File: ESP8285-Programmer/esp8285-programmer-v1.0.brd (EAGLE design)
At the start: 38.2 x 15.2 mm, 30 parts, among them J1 6p-2.54, J2 2p-2.54, J3 2p-2.54, K1 B3U-1000P, Q1 S9013, Q2 S9013, U1 CH340T-SSOP20, U2 CJA1117B-3.3-SOT89, Y1 12MHZ

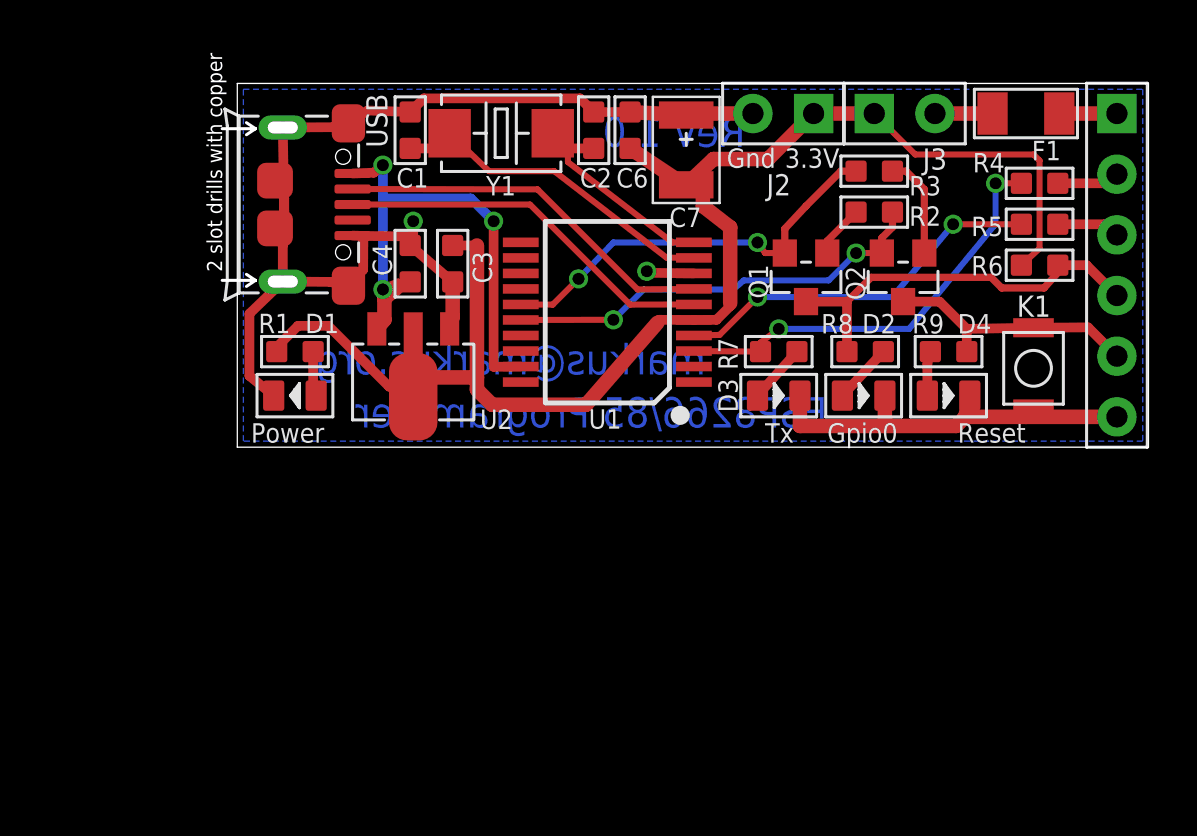
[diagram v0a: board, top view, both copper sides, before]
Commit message: Another Rev 1.0
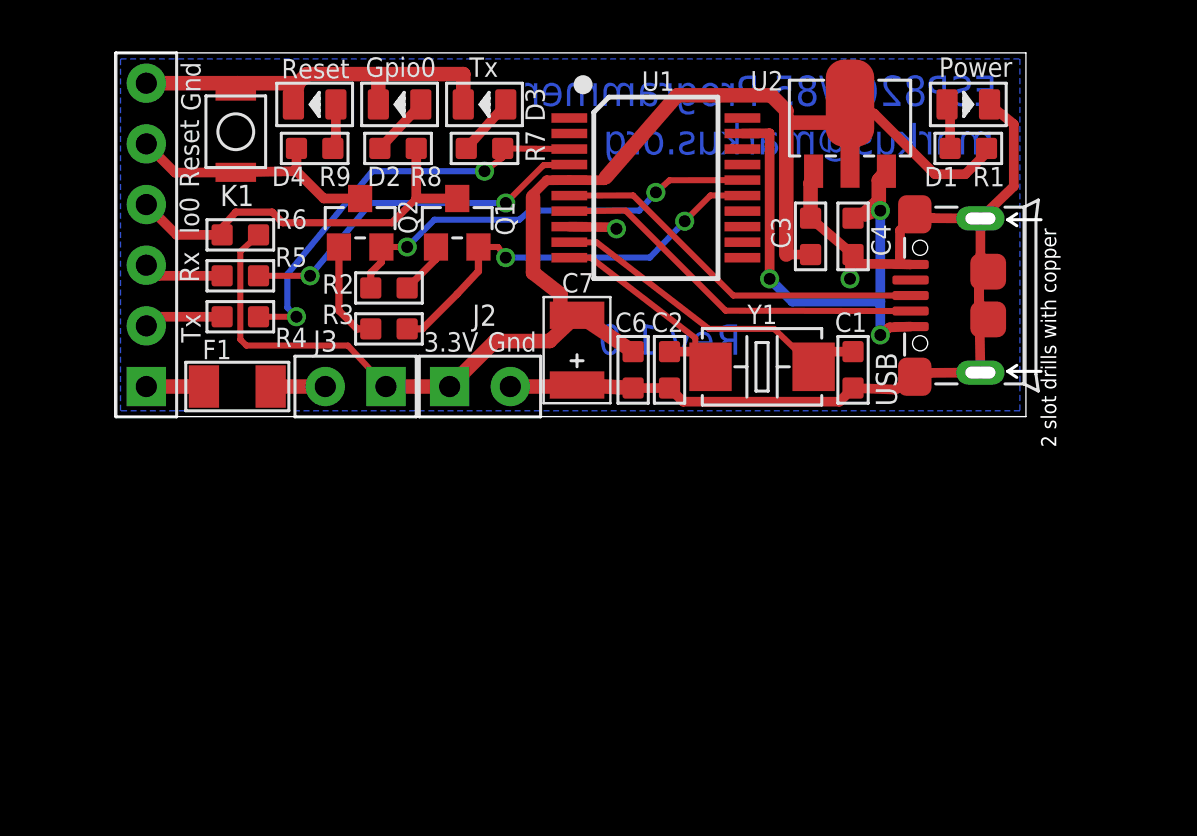
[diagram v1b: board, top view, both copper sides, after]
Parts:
- moved J1 40.7 mm to (2.54, 22.9), turned to 180 degrees
- moved F1 34.9 mm to (6.35, 16.5), turned to 0 degrees
- moved K1 34.8 mm to (6.29, 27.2), turned to 270 degrees
- moved R4 33.9 mm to (6.48, 19.4), turned to 270 degrees
- moved R5 33.5 mm to (6.48, 21.1), turned to 270 degrees
- moved R6 33.5 mm to (6.48, 22.9), turned to 270 degrees
- moved D1 30.7 mm to (37.0, 28.3), turned to 0 degrees
- moved R1 29.5 mm to (37.0, 26.5), turned to 90 degrees
- moved D4 29.2 mm to (9.59, 28.3), turned to 180 degrees
- moved R9 27.9 mm to (9.59, 26.5), turned to 270 degrees
- moved J3 25.7 mm to (11.3, 16.5), turned to 270 degrees
- moved USB 23.2 mm to (34.3, 20.3), turned to 90 degrees
- moved D2 22.9 mm to (13.1, 28.3), turned to 180 degrees
- moved Q2 22.8 mm to (11.5, 23.4), turned to 0 degrees
- moved R3 21.4 mm to (12.7, 18.9), turned to 90 degrees
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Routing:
- net N$15: track 2.64 -> 3.34 mm
- net N$14: track 2.59 -> 3.29 mm
- net N$RX: track 15.8 -> 15.1 mm
- net +3V3: track 63.0 -> 62.3 mm
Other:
- board text added: "Io0"
- board text added: "Rx"

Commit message: Hopefully final V1.0
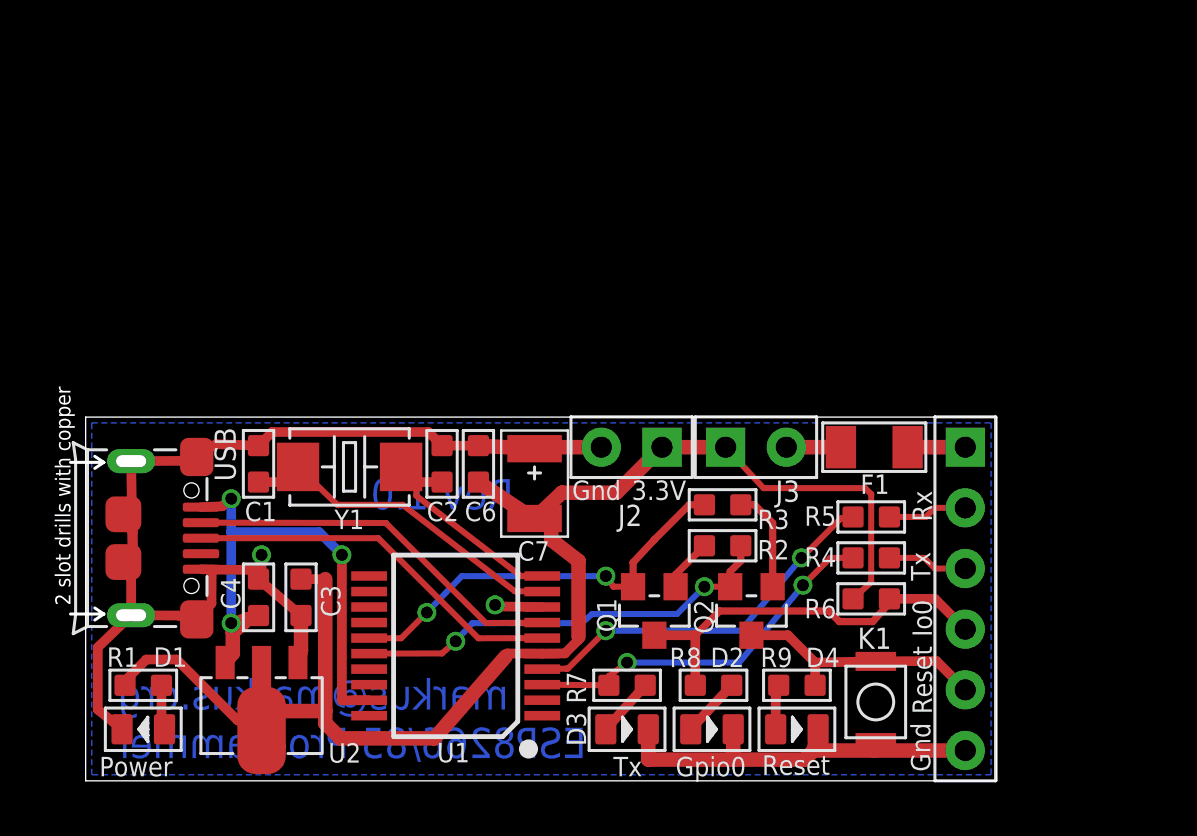
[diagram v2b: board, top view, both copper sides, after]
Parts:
- moved D1 43.3 mm to (2.41, 2.16), turned to 180 degrees
- moved R1 41.2 mm to (2.41, 4.00), turned to 270 degrees
- moved J1 37.5 mm to (36.8, 7.62), turned to 0 degrees
- moved K1 35.9 mm to (33.1, 3.30), turned to 90 degrees
- moved U2 34.7 mm to (7.37, 3.05), turned to 180 degrees
- moved D4 33.0 mm to (29.8, 2.16), turned to 0 degrees
- moved USB 30.9 mm to (5.08, 10.2), turned to 270 degrees
- moved R6 30.5 mm to (32.9, 7.62), turned to 90 degrees
- moved R9 30.2 mm to (29.8, 4.00), turned to 90 degrees
- moved D2 29.3 mm to (26.2, 2.16), turned to 0 degrees
- moved C4 29.1 mm to (7.24, 7.68), turned to 0 degrees
- moved R4 28.3 mm to (32.9, 9.33), turned to 90 degrees
- moved R5 28.3 mm to (32.9, 11.0), turned to 90 degrees
- moved D3 26.8 mm to (22.7, 2.16), turned to 0 degrees
- moved F1 26.8 mm to (33.0, 14.0), turned to 180 degrees
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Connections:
- removed net N$14: J1.2, R4.2
- removed net N$15: J1.3, R5.2
- new net N$4: J1.2, R5.2
- new net N$7: J1.3, R4.2
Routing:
- net N$7: track 0.00 -> 3.36 mm
- net N$15: track 3.34 -> 0.00 mm
- net N$4: track 0.00 -> 3.33 mm
- net N$14: track 3.29 -> 0.00 mm
- net N$TX: track 17.9 -> 15.6 mm
- net N$RX: track 15.1 -> 15.8 mm
